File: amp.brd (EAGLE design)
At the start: 100 x 80 mm, 25 parts, among them IC1 TDA2030V

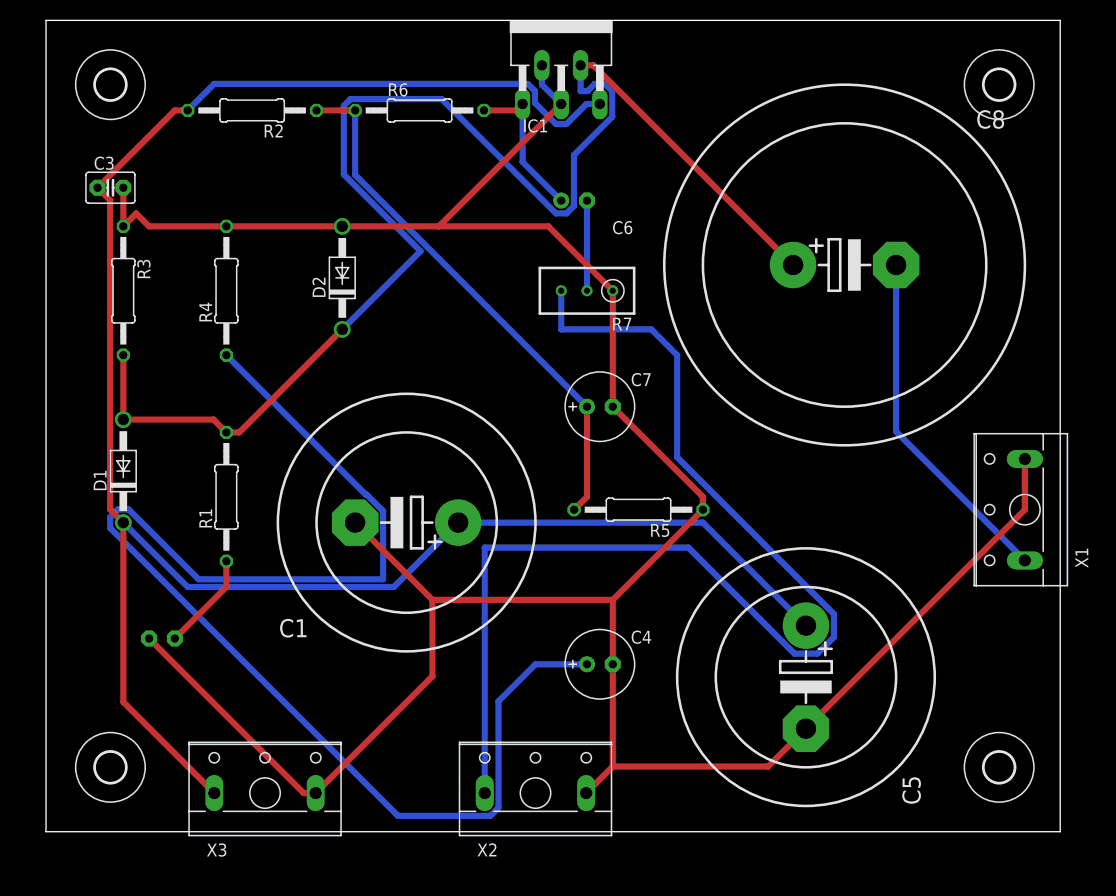
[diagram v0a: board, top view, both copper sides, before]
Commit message: Barna .brd ver2.0
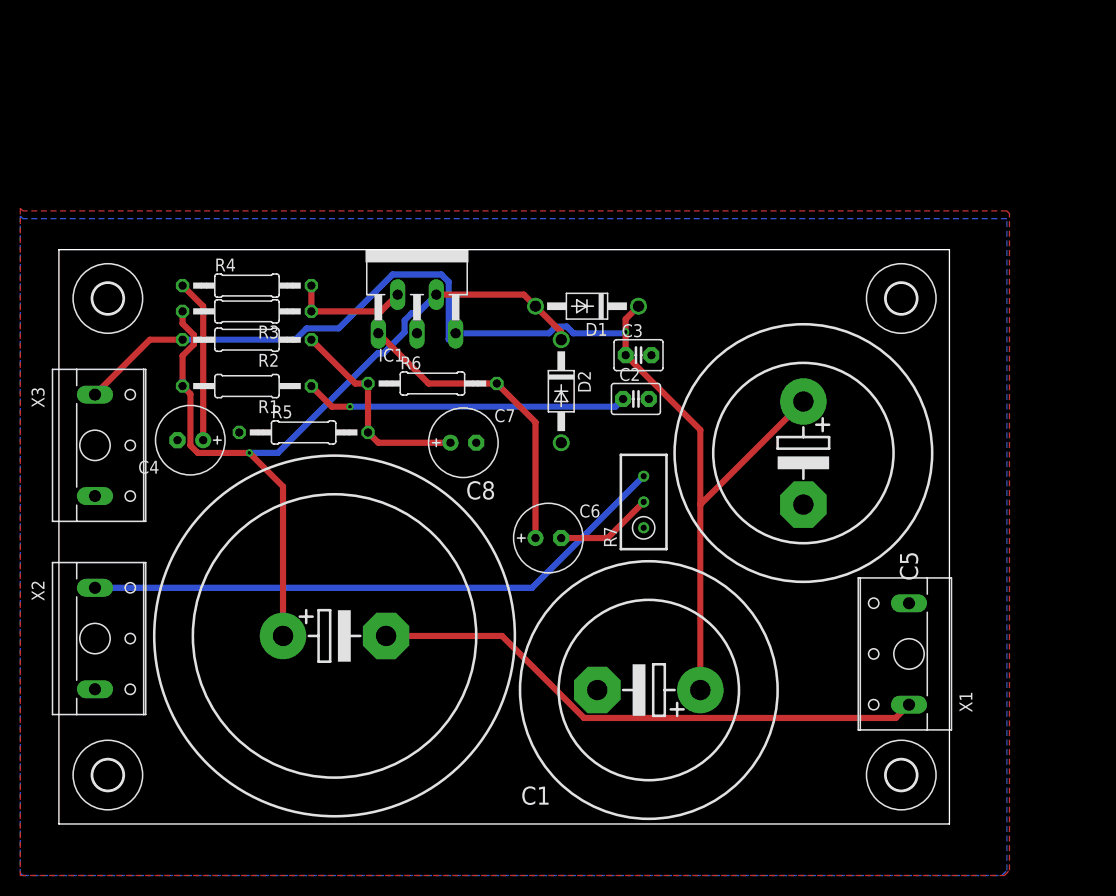
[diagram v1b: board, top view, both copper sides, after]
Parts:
- moved H3 103.5 mm to (84.3, 5.59)
- moved H2 99.3 mm to (6.10, 52.6)
- moved C8 62.2 mm to (28.4, 19.3)
- moved C3 54.6 mm to (58.4, 47.0)
- moved C2 52.4 mm to (58.2, 42.7), flipped to the top
- moved D1 48.5 mm to (53.3, 51.8), turned to 180 degrees
- moved C4 46.0 mm to (14.2, 38.6), turned to 180 degrees
- moved X2 44.4 mm to (6.10, 19.1), turned to 270 degrees
- moved X3 36.5 mm to (6.10, 38.1), turned to 270 degrees
- moved R5 33.9 mm to (25.4, 39.4), turned to 0 degrees
- moved C6 33.4 mm to (49.5, 29.0), flipped to the top, turned to 0 degrees
- moved C1 29.0 mm to (59.4, 14.0)
- moved R6 27.0 mm to (38.1, 44.2)
- moved IC1 26.7 mm to (36.6, 57.4)
- moved D2 24.3 mm to (50.8, 43.4), turned to 270 degrees
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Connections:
- new net N$7: IC1.2, R3.1, R4.2
- net GND: no longer IC1.2, R3.1, R4.2
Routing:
- net GND: track 266.6 -> 0.00 mm
- net N$1: track 130.8 -> 16.1 mm
- net VCC: track 198.1 -> 119.9 mm, vias 0 -> 1
- net N$4: track 137.2 -> 80.2 mm, vias 0 -> 1
- net VPP: track 114.1 -> 58.7 mm
- net N$6: track 53.2 -> 20.8 mm
- net N$5: track 9.72 -> 31.9 mm, vias 0 -> 1
- net N$2: track 34.4 -> 55.5 mm
- net N$3: track 15.2 -> 30.6 mm
- net N$7: track 0.00 -> 11.7 mm
- net N$9: track 8.89 -> 9.60 mm
- added copper zone on layer 1, net GND
- added copper zone on layer 16, net GND
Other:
- board size 100 x 80 mm -> 87.8 x 56.6 mm
